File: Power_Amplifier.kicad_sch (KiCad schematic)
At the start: 21 parts, among them Q1 BC547, Q2 2N3904

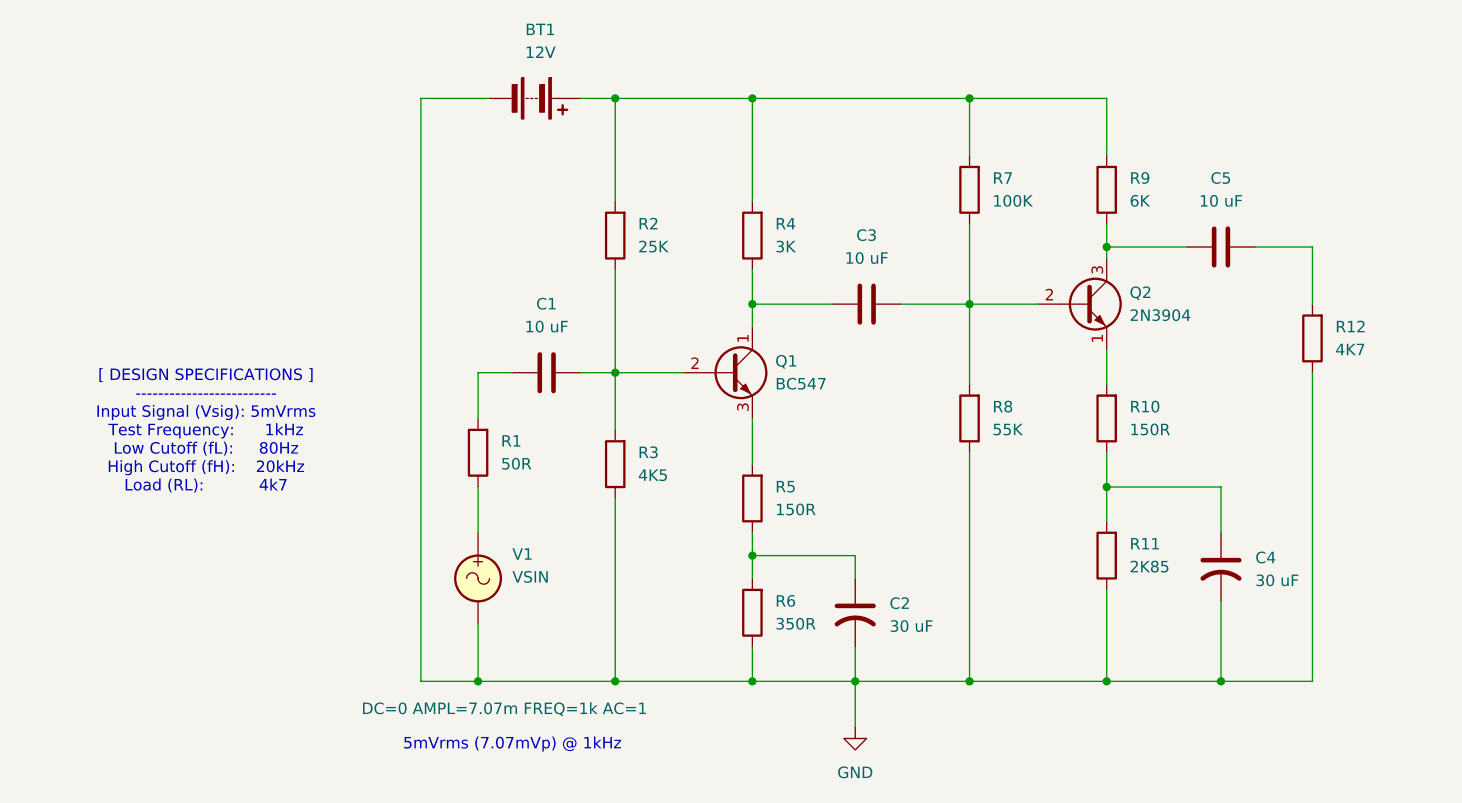
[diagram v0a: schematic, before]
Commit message: version 1.1: 2.26.2026
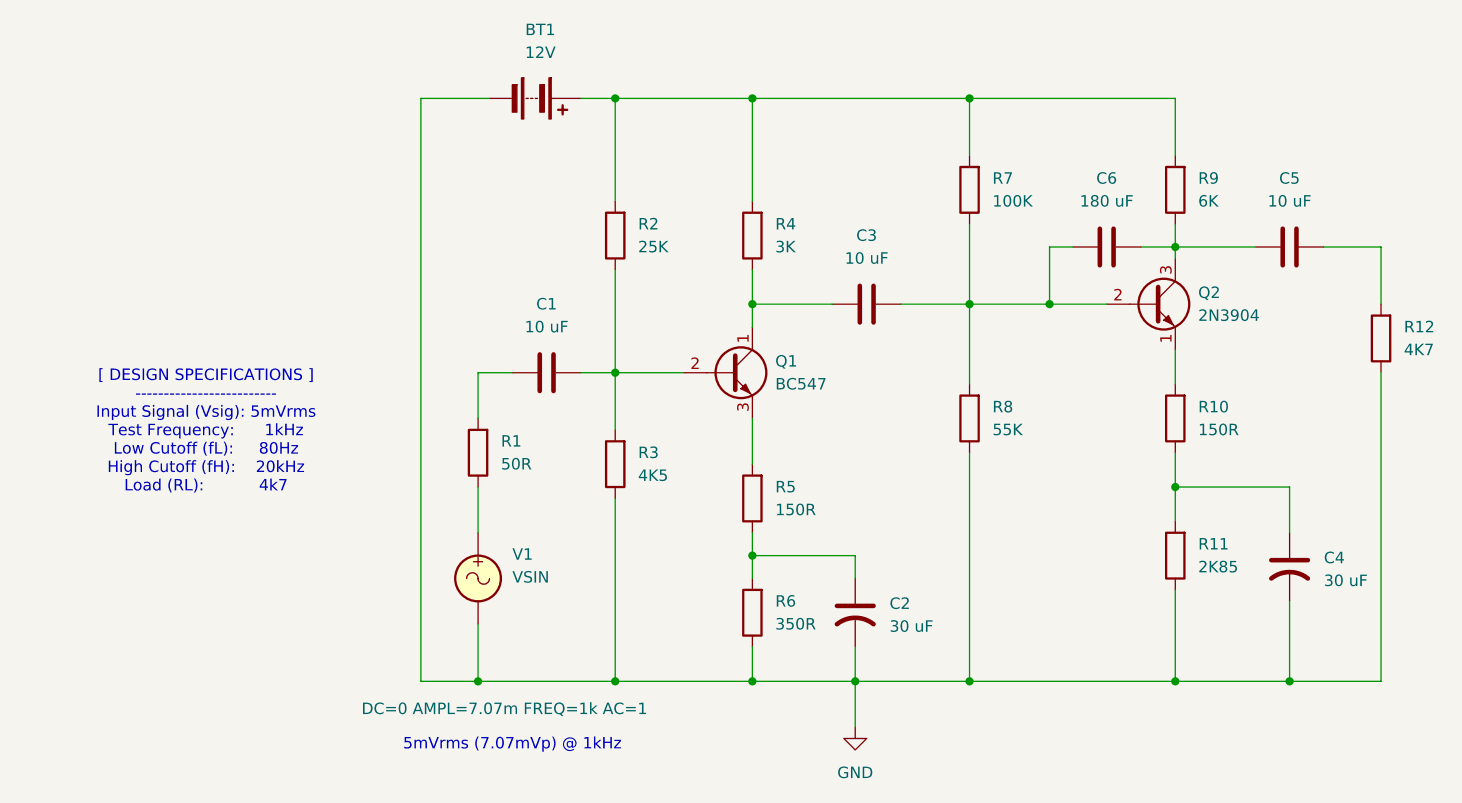
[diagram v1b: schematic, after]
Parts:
- added C6: 180 uF, Capacitor_THT:C_Disc_D4.3mm_W1.9mm_P5.00mm, symbol Device:C
- C1, C3, C5: footprint Capacitor_THT:C_Disc_D9.0mm_W5.0mm_P5.00mm -> Capacitor_THT:C_Disc_D5.1mm_W3.2mm_P5.00mm
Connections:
- net at C5.2, Q2.3 (C), R9.1: now also C6.1
- net at C3.2, Q2.2 (B), R7.1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: now also C6.2
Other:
- title: (none) -> Power Amplifier
- moved on the sheet: C4, C5, Q2, R10, R11, R12, R9
